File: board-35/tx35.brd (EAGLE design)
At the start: 100 x 80 mm, 23 parts, among them J1 SWD_SHROUD, Q1 MOSFET-NCHANNEL2N7002PW, X1 SMA-142-0711-821/826

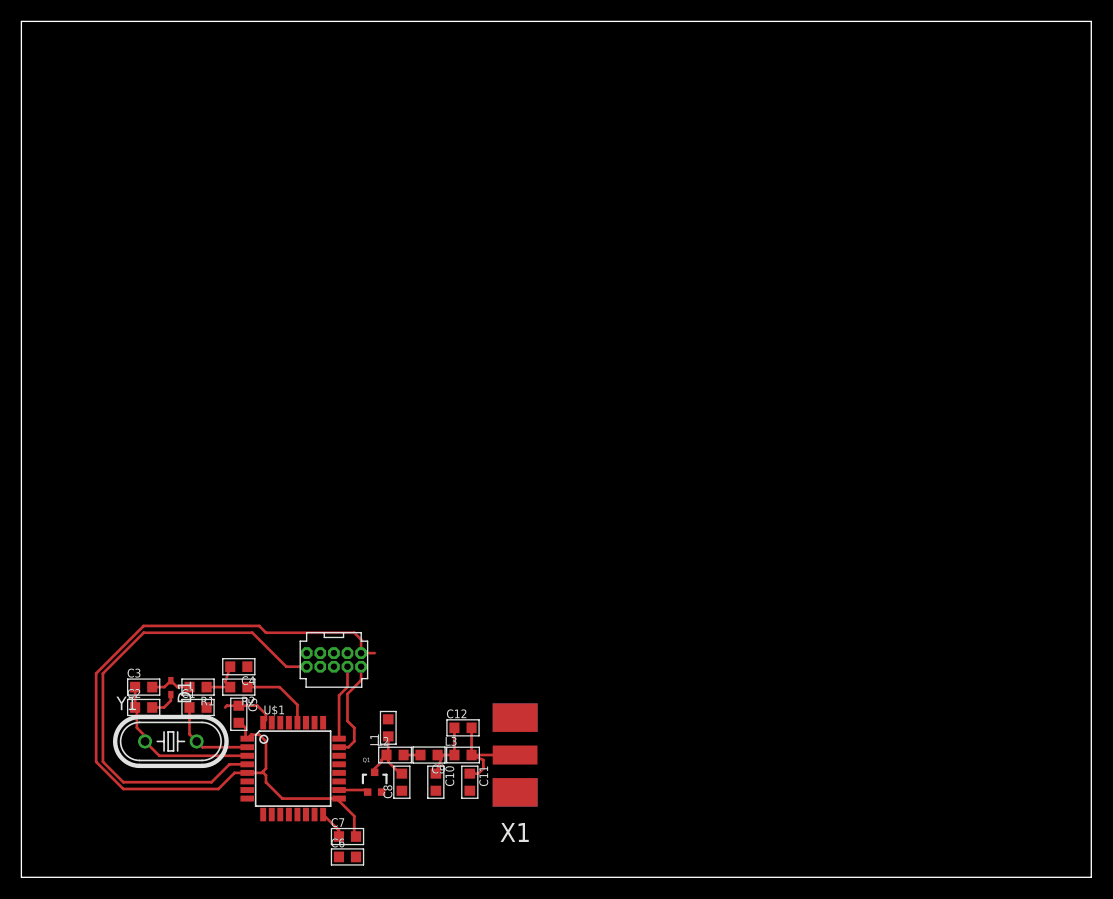
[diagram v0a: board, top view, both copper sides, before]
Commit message: almost done 35mhz tranasmitter
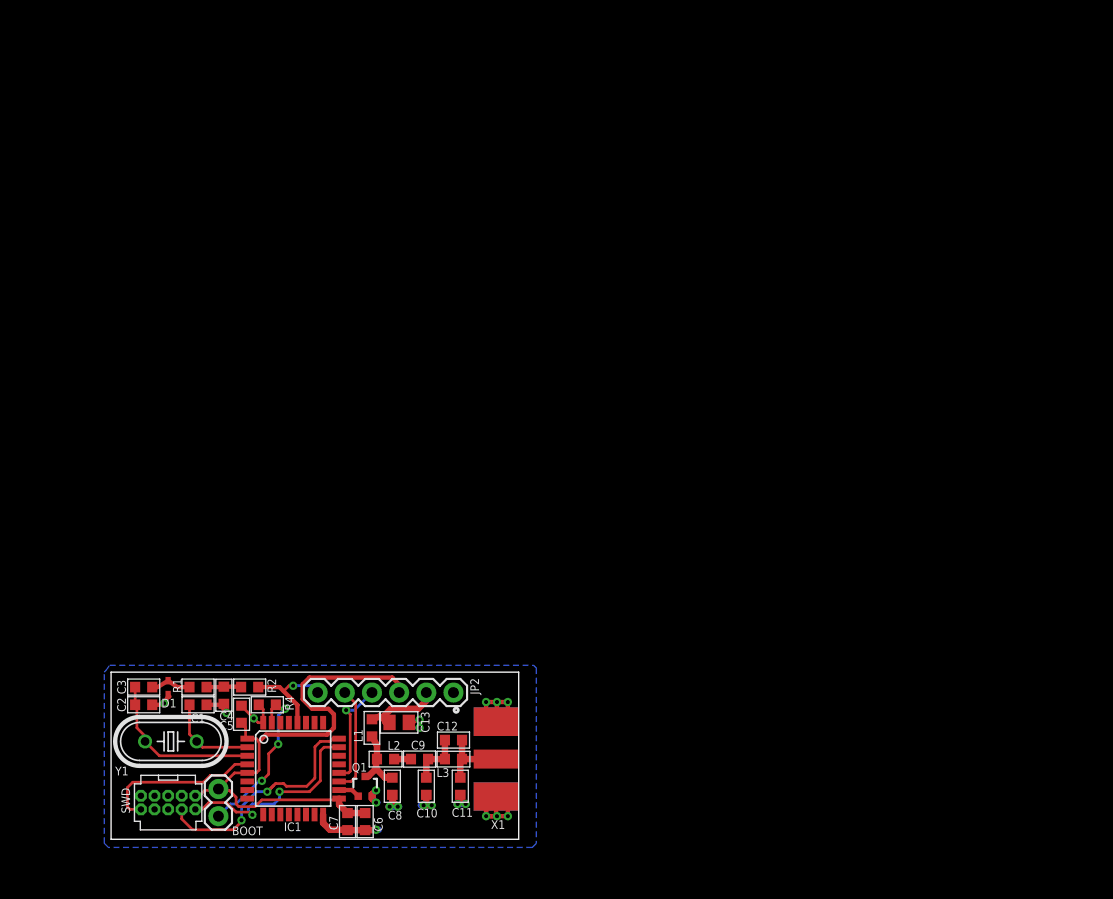
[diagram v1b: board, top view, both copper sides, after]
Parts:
- added C13: (no value), passives-7351:C0805-N
- added JP1: (no value), Mine:1X02
- added JP2: (no value), SparkFun-Connectors:1X06
- added R4: 10k, passives-7351:R0603-N
- IC1: value STM32F0-32 -> STM32F030K6
- moved J1 20.4 mm to (13.7, 6.99)
- moved C6 3.69 mm to (32.1, 5.21), turned to 90 degrees
- moved C4 3.01 mm to (18.9, 17.0), turned to 90 degrees
- moved X1 1.82 mm to (46.5, 11.0)
- moved L1 1.52 mm to (32.8, 14.0)
- moved C12 1.45 mm to (40.4, 12.8)
- moved C7 1.40 mm to (30.5, 5.21), turned to 90 degrees
- moved R2 1.02 mm to (21.3, 17.8)
- moved C10 0.97 mm to (37.8, 8.51)
- moved C8 0.97 mm to (34.7, 8.51)
- moved C9 0.97 mm to (37.2, 11.0)
- moved Q1 0.97 mm to (32.1, 8.51)
- moved C11 0.97 mm to (41.0, 8.51)
- moved L2 0.97 mm to (34.0, 11.0)
- moved L3 0.97 mm to (40.4, 11.0)
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- renumbered U$1 to IC1
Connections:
- new net N$12: IC1.19, JP2.5
- new net N$13: IC1.31, JP1.1, R4.1
- new net N$7: C13.1, JP2.2, L1.2
- new net N$9: IC1.20, JP2.4
- net +3V3: now also JP1.2, JP2.3
- net GND: now also C13.2, JP2.1, R4.2
- net N$5: now also JP2.6
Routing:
- net GND: track 10.3 -> 48.9 mm, vias 0 -> 20
- net NRST: track 45.2 -> 15.3 mm
- net +3V3: track 75.0 -> 52.6 mm
- net SWDCLK: track 7.05 -> 23.2 mm, vias 0 -> 2
- net N$13: track 0.00 -> 16.0 mm, vias 0 -> 3
- net SWDIO: track 9.42 -> 20.1 mm, vias 0 -> 2
- net N$9: track 0.00 -> 10.1 mm, vias 0 -> 1
- net N$12: track 0.00 -> 10.0 mm
- net N$7: track 0.00 -> 8.05 mm
- net N$6: track 10.1 -> 6.77 mm
- net N$5: track 7.03 -> 9.81 mm, vias 0 -> 1
- net N$4: track 4.38 -> 3.26 mm
- net N$8: track 5.97 -> 5.16 mm
- net MCO: track 2.76 -> 2.03 mm
- added copper zone on layer 16, net GND
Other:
- board size 100 x 80 mm -> 38.1 x 15.6 mm
- board text added: "3.3V"
- board text added: "BOOT"
- board text added: "EN"
- board text added: "GND"
- board text added: "HF Transmitter"
- board text added: "Jan 2016"
- board text added: "MOD_IN"
- board text added: "Matt Brejza"
- board text added: "SWD"
- board text added: "UART_RX"
- board text added: "V_PA"
